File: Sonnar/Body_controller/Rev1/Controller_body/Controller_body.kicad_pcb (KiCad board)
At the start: 2 copper layers, 40.6 x 79 mm, 23 parts, among them J1 Conn_01x06_Socket, J2 Conn_01x03_Socket, U1 PCF8575PWR

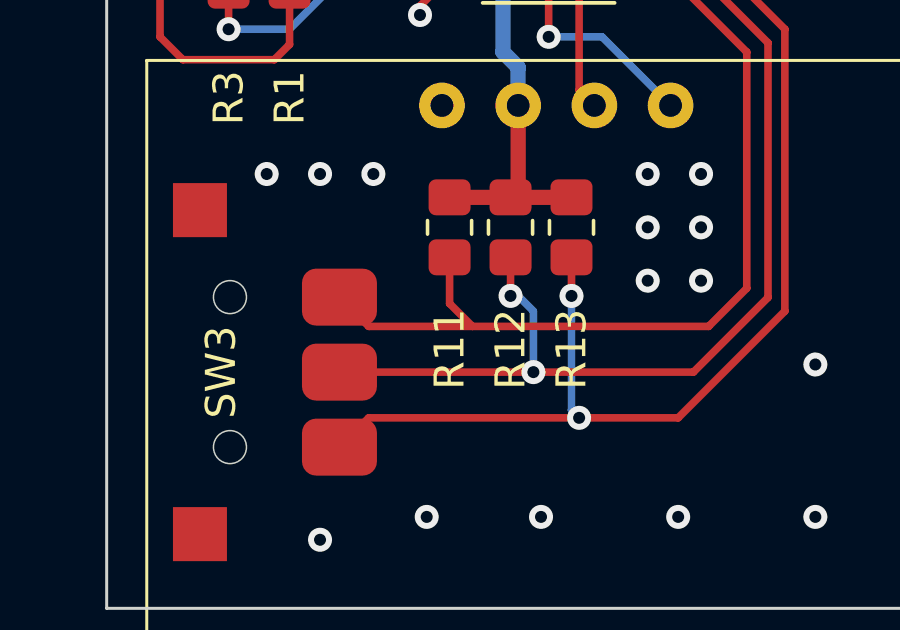
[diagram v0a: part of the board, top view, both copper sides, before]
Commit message: code upgrade
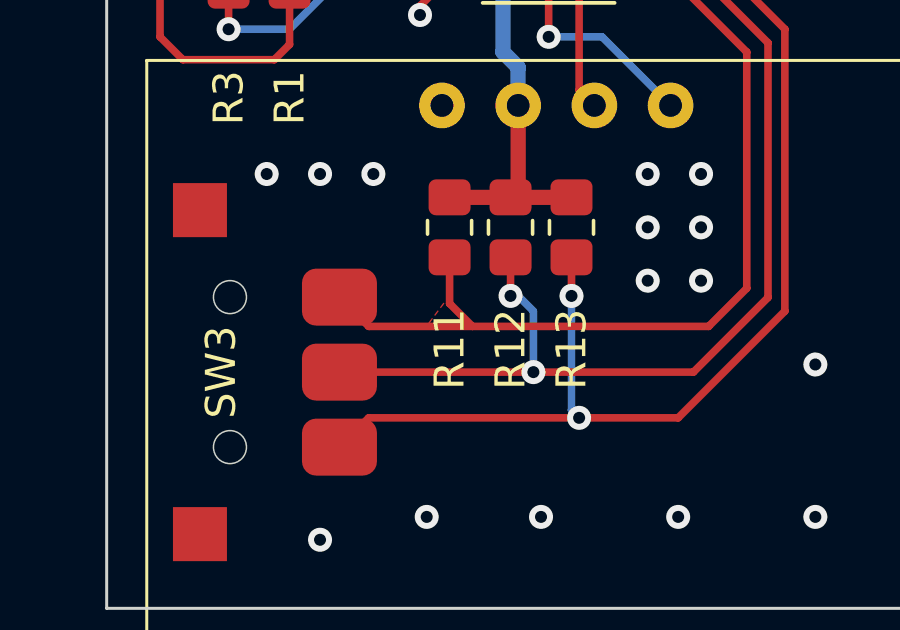
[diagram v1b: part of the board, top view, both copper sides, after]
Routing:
- added copper zone on F.Cu, net /SW_B
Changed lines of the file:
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@@
+    )
+  )
+  (zone (net 23) (net_name "/SW_B") (layer "F.Cu") (hatch edge 0.5)
+    (priority 3)
+    (connect_pads (clearance 0.7))
+    (min_thickness 0.25) (filled_areas_thickness no)
+    (fill yes (thermal_gap 0.5) (thermal_bridge_width 0.5))
+    (polygon
+      (pts
+        (xy 91.3 118.6)
+        (xy 91 118.6)
+        (xy 90.4 119.4)
+        (xy 92 119.4)
+      )
     )
   )
